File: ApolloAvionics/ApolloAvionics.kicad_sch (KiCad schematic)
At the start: 3 parts, among them U1 BMP388, U2 MPU-6000

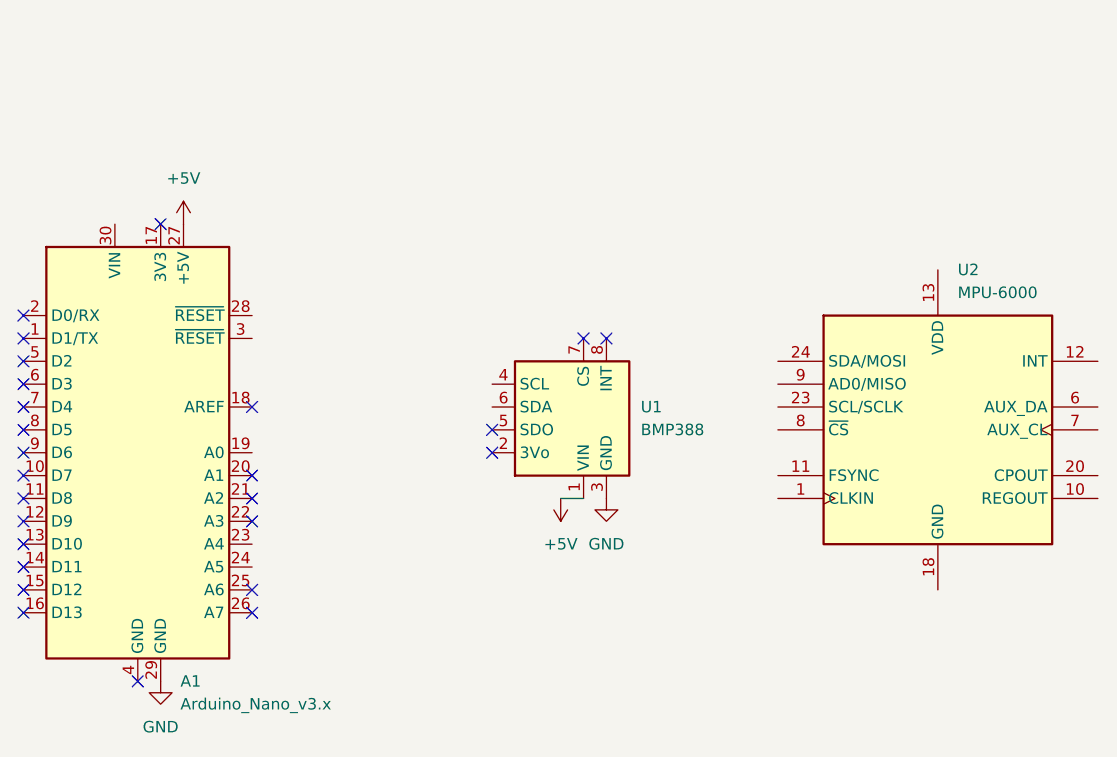
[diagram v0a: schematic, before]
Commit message: Sensor schematics
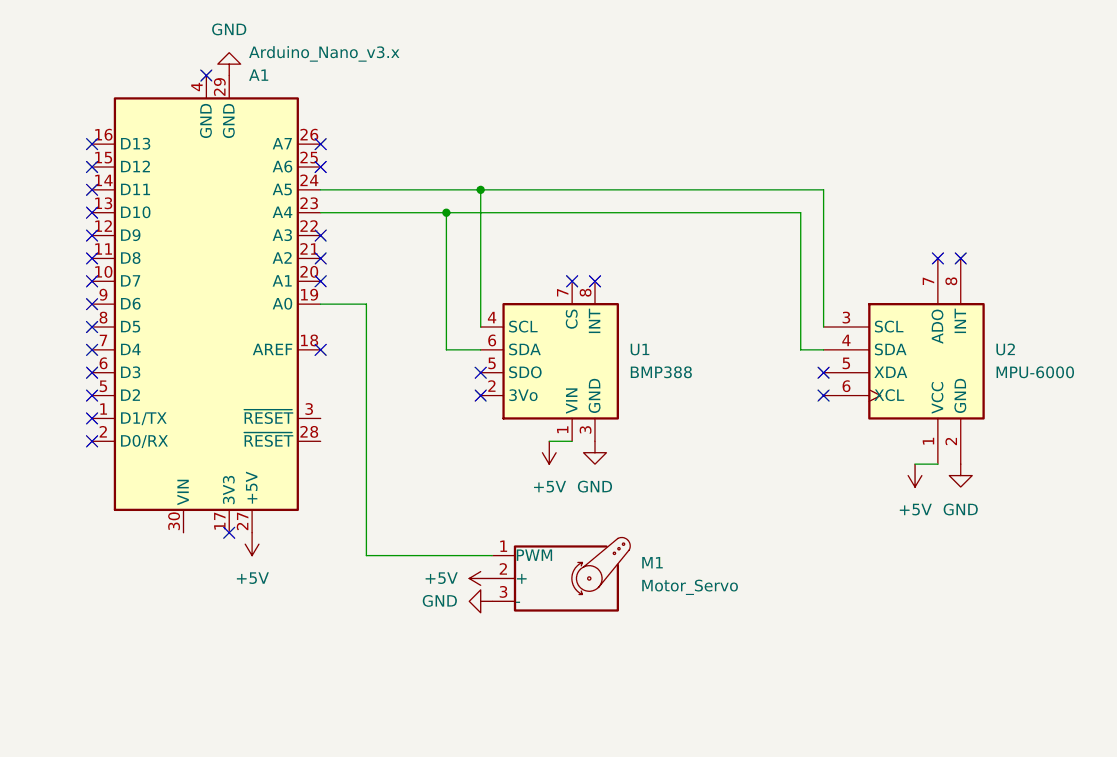
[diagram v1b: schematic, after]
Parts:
- added M1: Motor_Servo, symbol Motor:Motor_Servo
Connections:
- net +5V: now also U2.1 (VCC), M1.2 (+)
- net GND: now also U2.2 (GND), M1.3 (-)
- net at A1.19 (A0): now also M1.1 (PWM)
- net at A1.23 (A4): now also U1.6 (SDA), U2.4 (SDA)
- net at A1.24 (A5): now also U1.4 (SCL), U2.3 (SCL)
- no-connect marks 26 -> 30
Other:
- moved on the sheet: A1, U1
